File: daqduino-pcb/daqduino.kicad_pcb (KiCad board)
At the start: 2 copper layers, 68.6 x 53.3 mm, 39 parts, among them J1 24v Power Input, J2 Sense Current TestPoint, J3 Bias Voltage & Resistor Selec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, J4 Sensor Voltage Selection, J5 2 Wire Sensor (4-20mA), J7 Micro_SD_Card-molex, U1 LM358, U2 L7812, U3 TXS0108EPW

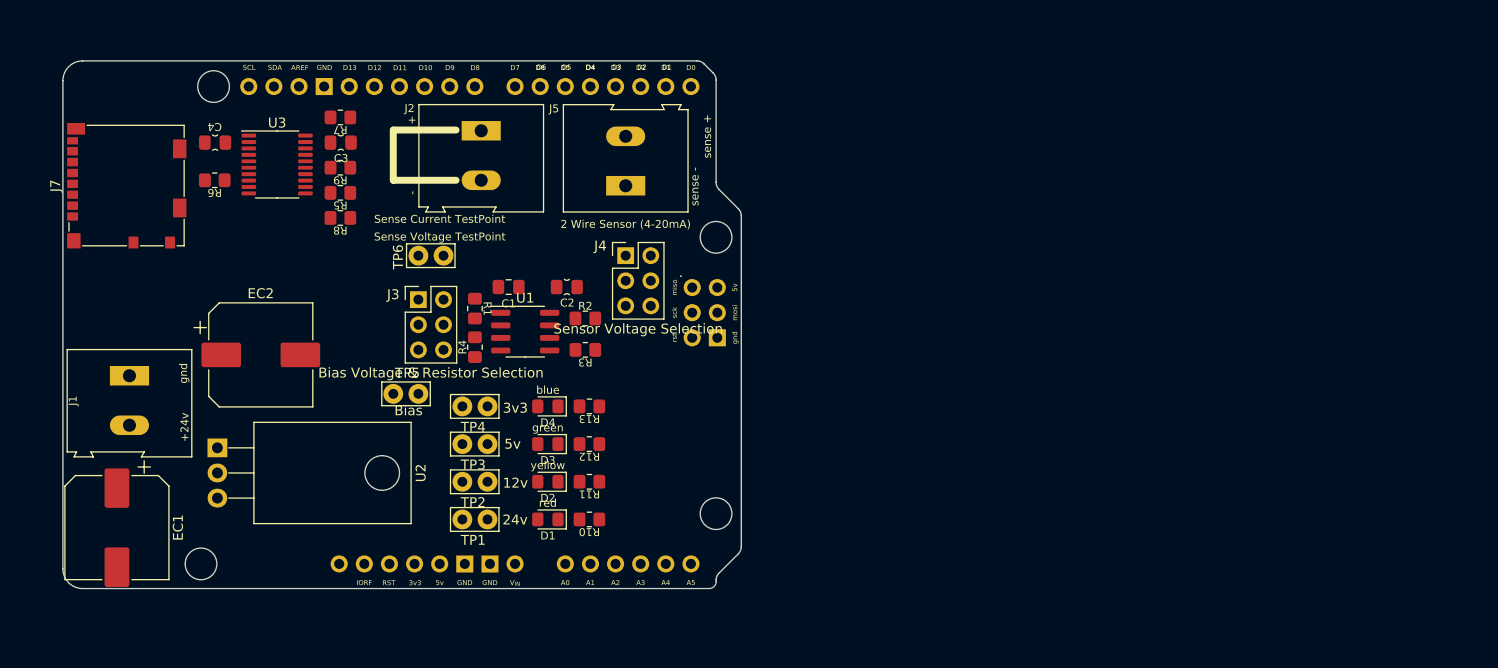
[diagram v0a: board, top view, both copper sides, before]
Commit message: finished PCB design
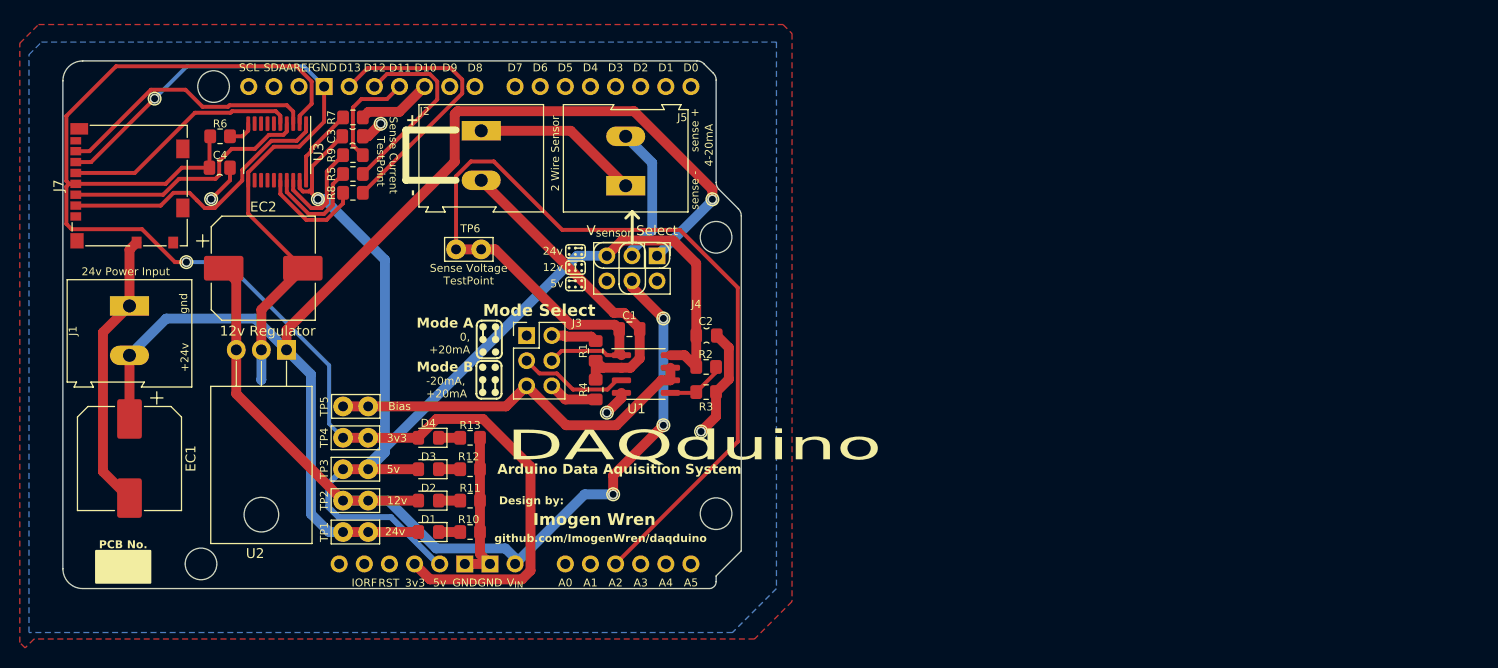
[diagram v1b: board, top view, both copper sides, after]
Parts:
- C1: value 470r -> 470n
- J2: value Sense Current TestPoint -> Sense Current
- J3: value Bias Voltage & Resistor Selection -> Mode Select
- J4: value Sensor Voltage Selection -> V_{sensor} Select
- J5: value 2 Wire Sensor (4-20mA) -> 2 Wire Sensor
- J7: value Micro_SD_Card-molex -> Micro SD Card
- TP6: value Sense Voltage TestPoint -> Sense Voltage
- U2: value L7812 -> 12v Regulator
- XA1: value Arduino_Uno_R3_Shield -> Arduino_Uno_R3_Shield-simple; footprint PCM_arduino-library:Arduino_Uno_R3_Shield -> 000_Modules_Immo:Arduino_Uno_R3_Shield-simple
- moved C2 14.9 mm to (124.4, 72.2)
- moved R2 13.2 mm to (124.3, 75.4), turned to 180 degrees
- moved U1 12.9 mm to (118.3, 76.1)
- moved R1 12.9 mm to (113.2, 73.8)
- moved R4 12.9 mm to (113.2, 77.7)
- moved R3 12.9 mm to (124.3, 77.9)
- moved C1 12.9 mm to (116.6, 71.6)
- moved R13 12.5 mm to (100.5, 82.5)
- moved D4 12.5 mm to (96.3, 82.5)
- moved TP4 12.5 mm to (87.6, 82.5)
- moved R12 12.3 mm to (100.5, 85.7)
- moved D3 12.3 mm to (96.3, 85.7)
- moved TP3 12.3 mm to (87.6, 85.7)
- moved R11 12.2 mm to (100.5, 88.9)
- moved D2 12.2 mm to (96.3, 88.9)
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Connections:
- J7 pad 11: unconnected-(J7-n/c-Pad11) -> (no net)
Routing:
- net /3V3_BUS: track 0.00 -> 146.8 mm, vias 0 -> 1
- net GND: track 0.00 -> 135.2 mm, vias 0 -> 5
- net /5V_BUS: track 0.00 -> 126.2 mm, vias 0 -> 1
- net /24V_BUS: track 0.00 -> 123.7 mm, vias 0 -> 1
- net /R_SET_B: track 0.00 -> 105.0 mm
- net /12V_BUS: track 0.00 -> 94.3 mm, vias 0 -> 3
- net Net-(J3-Pin_3): track 0.00 -> 38.8 mm
- net /R_SET_A: track 0.00 -> 32.2 mm
- net /CS: track 0.00 -> 29.1 mm
- net /SCK: track 0.00 -> 28.3 mm
- net /D_{OUT}: track 0.00 -> 26.8 mm
- net /D_{IN}: track 0.00 -> 25.6 mm
- net /CLK: track 0.00 -> 24.3 mm
- net /MOSI: track 0.00 -> 19.7 mm
- net /SENSE_CURRENT: track 0.00 -> 16.9 mm
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- added copper zone on B.Cu, net GND
- added copper zone on F.Cu, net GND
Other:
- outline, holes or cut-outs redrawn
- board text added: "-20mA, +20mA"
- board text added: "0, +20mA"
- board text added: "12v"
- board text added: "24v"
- board text added: "4-20mA"
- board text added: "5v"
- board text added: "Arduino Data Aquisition System"
- board text added: "DAQduino"
- board text added: "Design by:"
- board text added: "Imogen Wren"
- board text added: "Mode A"
- board text added: "Mode B"
- board text added: "PCB No."
- board text added: "TestPoint"
- board text added: "github.com/ImogenWren/daqduino"
- board text removed: "D0"
- board text removed: "D1"
- board text removed: "D2"
- board text removed: "D3"
- board text removed: "D4"
- board text removed: "D5"
- board text removed: "D6"

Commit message: oshldgf
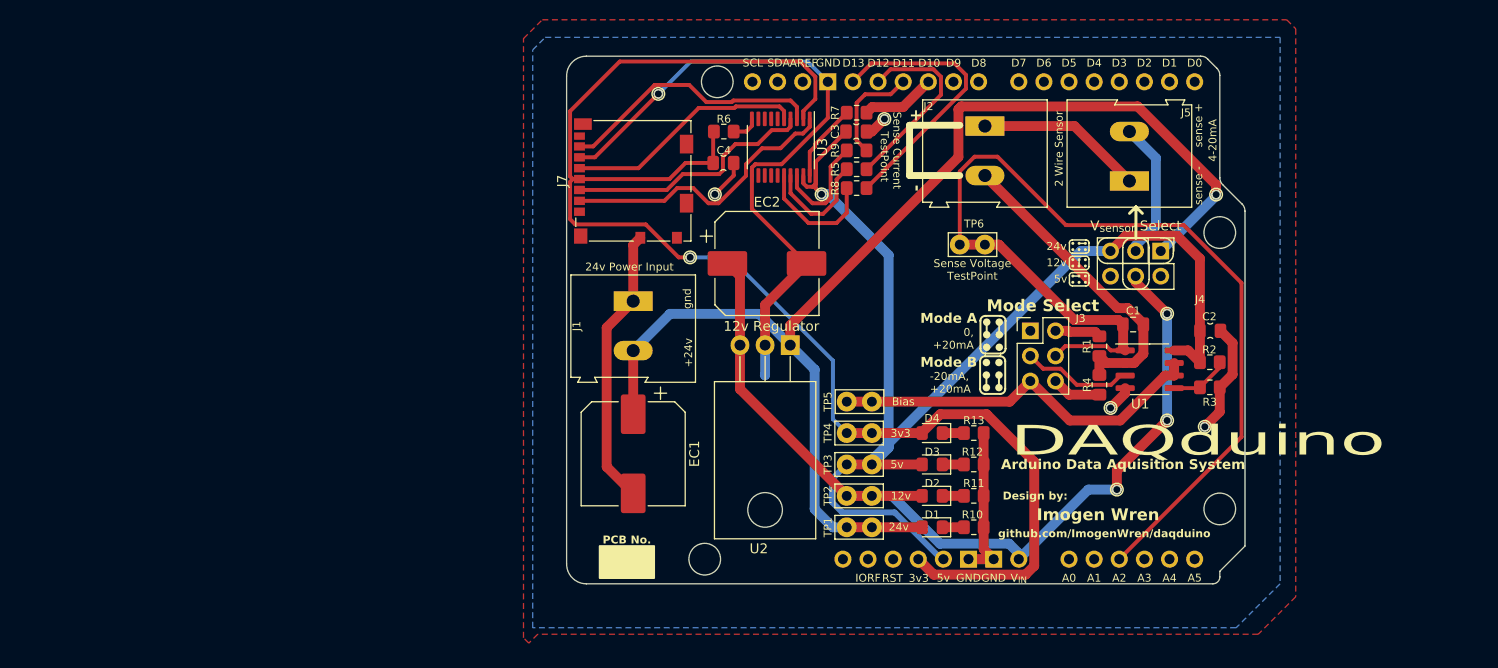
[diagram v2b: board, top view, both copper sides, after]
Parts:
- moved EC2 50.9 mm to (130.5, 64.9)
- moved J2 50.9 mm to (152.5, 51.0)
- moved R1 50.9 mm to (164.1, 73.3)
- moved R10 50.9 mm to (151.4, 91.6)
- moved R11 50.9 mm to (151.4, 88.4)
- moved R12 50.9 mm to (151.4, 85.2)
- moved R13 50.9 mm to (151.4, 82.1)
- moved R4 50.9 mm to (164.1, 77.2)
- moved R5 50.9 mm to (139.6, 55.4)
- moved R7 50.9 mm to (139.6, 49.7)
- moved R8 50.9 mm to (139.6, 57.3)
- moved R9 50.9 mm to (139.6, 53.5)
- moved TP1 50.9 mm to (138.6, 91.6)
- moved TP2 50.9 mm to (138.6, 88.4)
- moved TP3 50.9 mm to (138.6, 85.2)
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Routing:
- net Net-(U3-B4): track 10.6 -> 12.6 mm
- net Net-(U3-B3): track 10.7 -> 11.5 mm
